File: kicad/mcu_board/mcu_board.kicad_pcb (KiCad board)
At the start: 2 copper layers, 59.6 x 64.4 mm, 31 parts, among them J1 Buttons

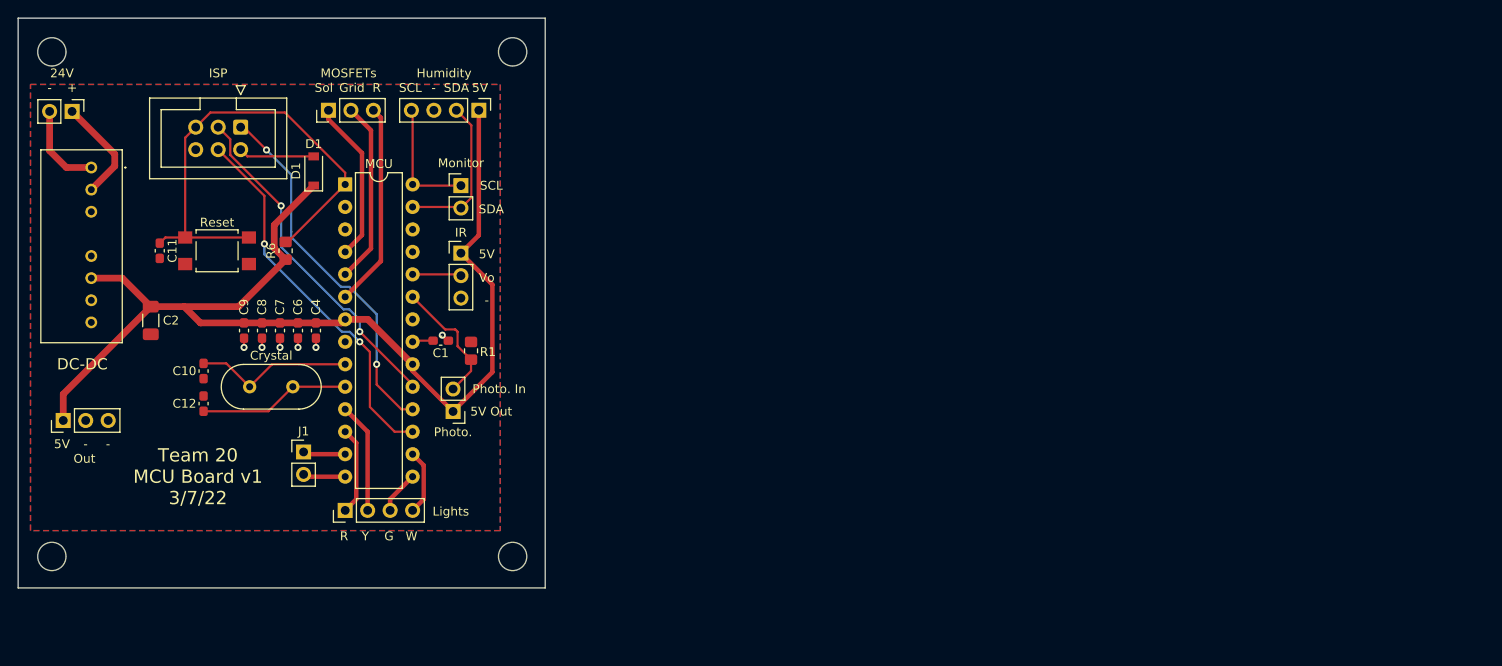
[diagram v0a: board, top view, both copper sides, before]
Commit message: finishing up MCU and adding gerbers
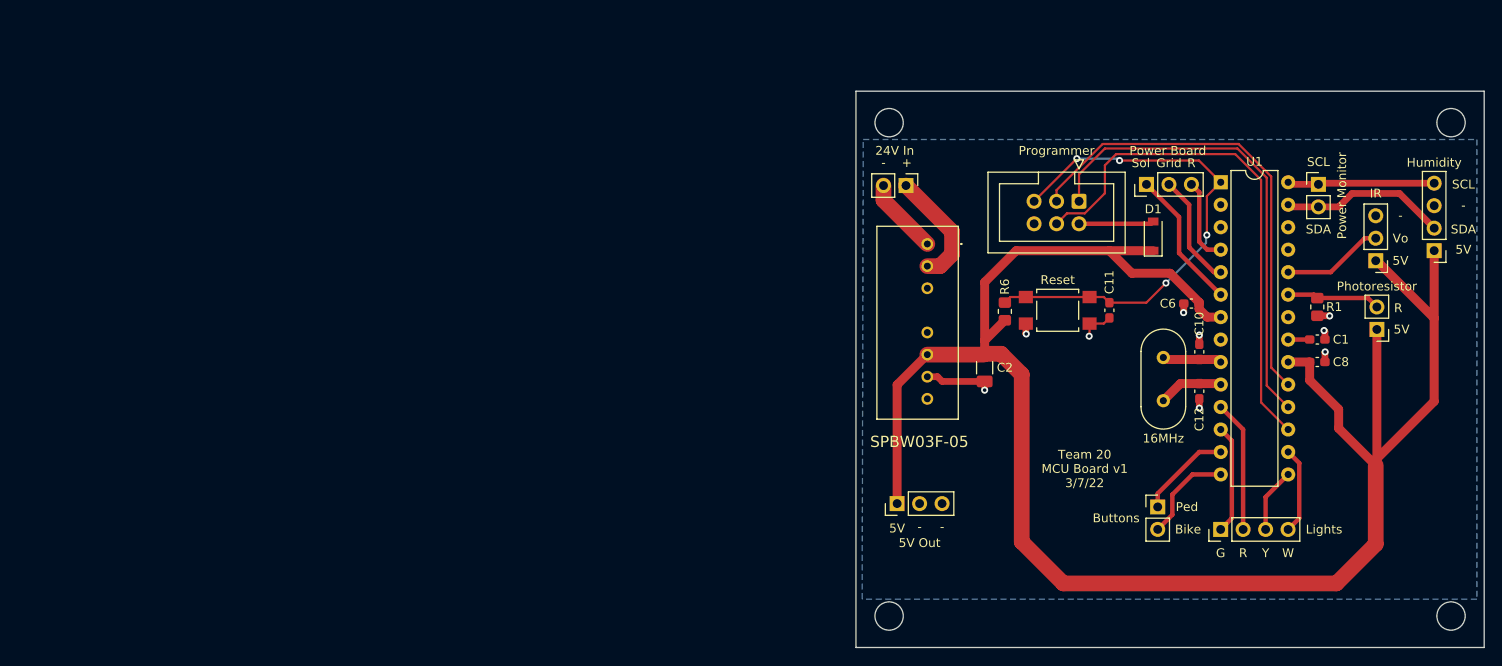
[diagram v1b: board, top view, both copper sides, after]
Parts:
- removed 24V: 24V In, Connector_PinHeader_2.54mm:PinHeader_1x02_P2.54mm_Vertical
- removed C4, C7, C9: 0.1uF, Capacitor_SMD:C_0603_1608Metric_Pad1.08x0.95mm_HandSolder
- removed Crystal: 16MHz, Crystal:Crystal_HC49-U_Vertical
- removed DC-DC: SPBW03F-05, SamacSys_Parts:SPBW06F05
- removed Humidity: Humidity, Connector_PinHeader_2.54mm:PinHeader_1x04_P2.54mm_Vertical
- removed IR: IR, Connector_PinHeader_2.54mm:PinHeader_1x03_P2.54mm_Vertical
- removed ISP: Programmer, Connector_IDC:IDC-Header_2x03_P2.54mm_Vertical
- removed Lights: Lights, Connector_PinHeader_2.54mm:PinHeader_1x04_P2.54mm_Vertical
- removed MCU: ATmega328-P, Package_DIP:DIP-28_W7.62mm
- removed Monitor: Power Monitor, Connector_PinHeader_2.54mm:PinHeader_1x02_P2.54mm_Vertical
- removed Out: 5V Out, Connector_PinHeader_2.54mm:PinHeader_1x03_P2.54mm_Vertical
- removed Photo.: Photoresistor, Connector_PinHeader_2.54mm:PinHeader_1x02_P2.54mm_Vertical
- removed Reset: Reset, Button_Switch_SMD:SW_SPST_TL3305B
- removed Sol: Power Board, Connector_PinHeader_2.54mm:PinHeader_1x03_P2.54mm_Vertical
- added J10: Lights, Connector_PinHeader_2.54mm:PinHeader_1x04_P2.54mm_Vertical, F.Cu at (230.8, 132.1)
- added J2: Humidity, Connector_PinHeader_2.54mm:PinHeader_1x04_P2.54mm_Vertical, F.Cu at (254.9, 100.6)
- added J3: IR, Connector_PinHeader_2.54mm:PinHeader_1x03_P2.54mm_Vertical, F.Cu at (248.3, 101.7)
- added J4: Power Monitor, Connector_PinHeader_2.54mm:PinHeader_1x02_P2.54mm_Vertical, F.Cu at (241.8, 93.1)
- added J5: Photoresistor, Connector_PinHeader_2.54mm:PinHeader_1x02_P2.54mm_Vertical, F.Cu at (248.4, 109.5)
- added J6: 24V In, Connector_PinHeader_2.54mm:PinHeader_1x02_P2.54mm_Vertical, F.Cu at (195.2, 93.2)
- added J7: 5V Out, Connector_PinHeader_2.54mm:PinHeader_1x03_P2.54mm_Vertical, F.Cu at (194.2, 129.2)
- added J8: Programmer, Connector_IDC:IDC-Header_2x03_P2.54mm_Vertical, F.Cu at (214.8, 95.0)
- added J9: Power Board, Connector_PinHeader_2.54mm:PinHeader_1x03_P2.54mm_Vertical, F.Cu at (222.4, 93.1)
- added PS1: SPBW03F-05, SamacSys_Parts:SPBW06F05, F.Cu at (197.6, 99.8)
- added SW1: Reset, Button_Switch_SMD:SW_SPST_TL3305B, F.Cu at (212.3, 107.3)
- added U1: ATmega328-P, Package_DIP:DIP-28_W7.62mm, F.Cu at (230.8, 92.8)
- added Y1: 16MHz, Crystal:Crystal_HC49-U_Vertical, F.Cu at (224.3, 112.6)
- moved C8 119.3 mm to (241.7, 113.2), turned to 0 degrees
- moved C10 112.5 mm to (228.3, 112.0), turned to 90 degrees
- moved C12 112.5 mm to (228.3, 116.5), turned to -90 degrees
- moved C11 107.5 mm to (218.2, 107.3)
- moved H3 106.3 mm to (256.8, 86.1)
- moved H4 106.3 mm to (256.8, 141.9)
- moved C6 101.0 mm to (227.5, 106.5), turned to 180 degrees
- moved C1 99.1 mm to (241.7, 110.6)
- moved J1 96.7 mm to (223.6, 129.5)
- moved R1 95.8 mm to (241.7, 106.9), turned to -90 degrees
- moved D1 95.2 mm to (223.1, 98.9)
- moved H1 95.0 mm to (193.3, 86.1)
- moved H2 94.9 mm to (193.3, 141.9)
- moved C2 94.4 mm to (204.1, 113.8)
- moved R6 81.6 mm to (206.4, 107.4)
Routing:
- net +5V: track 127.5 -> 217.6 mm
- net MCU_MOSI: track 42.7 -> 58.9 mm, vias 2 -> 0
- net MCU_SCK: track 38.8 -> 53.5 mm, vias 2 -> 0
- net GND1: track 6.15 -> 19.5 mm, vias 6 -> 9
- net MCU_MISO: track 41.4 -> 53.7 mm, vias 2 -> 0
- net MCU_XTAL1: track 18.1 -> 6.70 mm
- net MCU_XTAL2: track 17.1 -> 7.33 mm
- net Solar: track 18.4 -> 9.64 mm
- net Grid: track 20.7 -> 12.8 mm
- net Resistor: track 23.1 -> 15.9 mm
- net Bike: track 4.80 -> 11.0 mm
- net Vo: track 5.52 -> 11.5 mm
- net Pedestrian: track 4.80 -> 10.6 mm
- net Photoresistor: track 14.7 -> 10.6 mm
- net MCU_N_RESET: track 54.4 -> 57.8 mm, vias 0 -> 4
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- removed copper zone on F.Cu, net GND1
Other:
- board size 59.6 x 64.4 mm -> 71 x 62.9 mm
- board text removed: "+"
- board text removed: "-"
- board text removed: "5V"
- board text removed: "5V Out"
- board text removed: "G"
- board text removed: "Grid"
- board text removed: "MOSFETs"
- board text removed: "Photo. In"
- board text removed: "R"
- board text removed: "SCL"
- board text removed: "SDA"
- board text removed: "Vo"
- board text removed: "W"
- board text removed: "Y"
